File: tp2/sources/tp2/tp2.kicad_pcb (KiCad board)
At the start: 2 copper layers, 61.5 x 42 mm, 34 parts, among them Q1 NPN, U1 LM324, U7 LM324

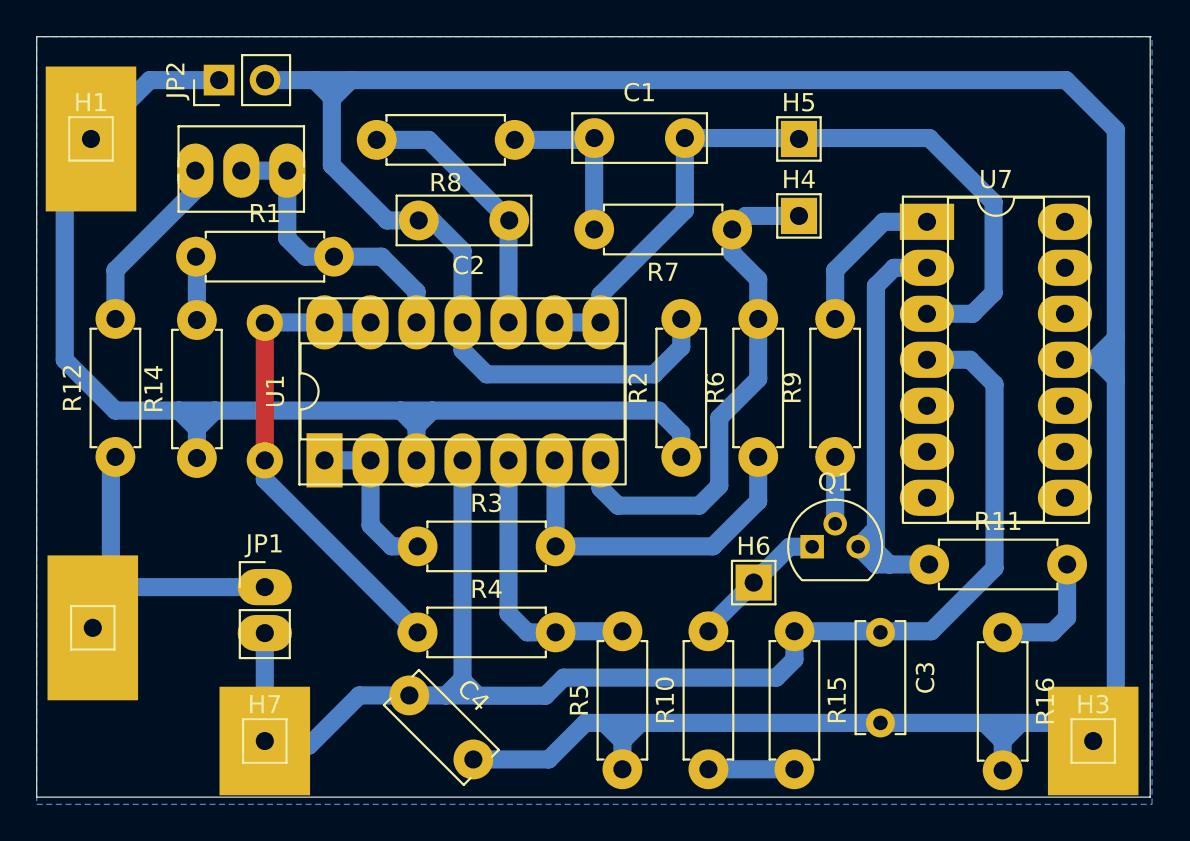
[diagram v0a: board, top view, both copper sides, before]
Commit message: tp2: achica 0.5mm (cero punto cinco milimietros) la placa
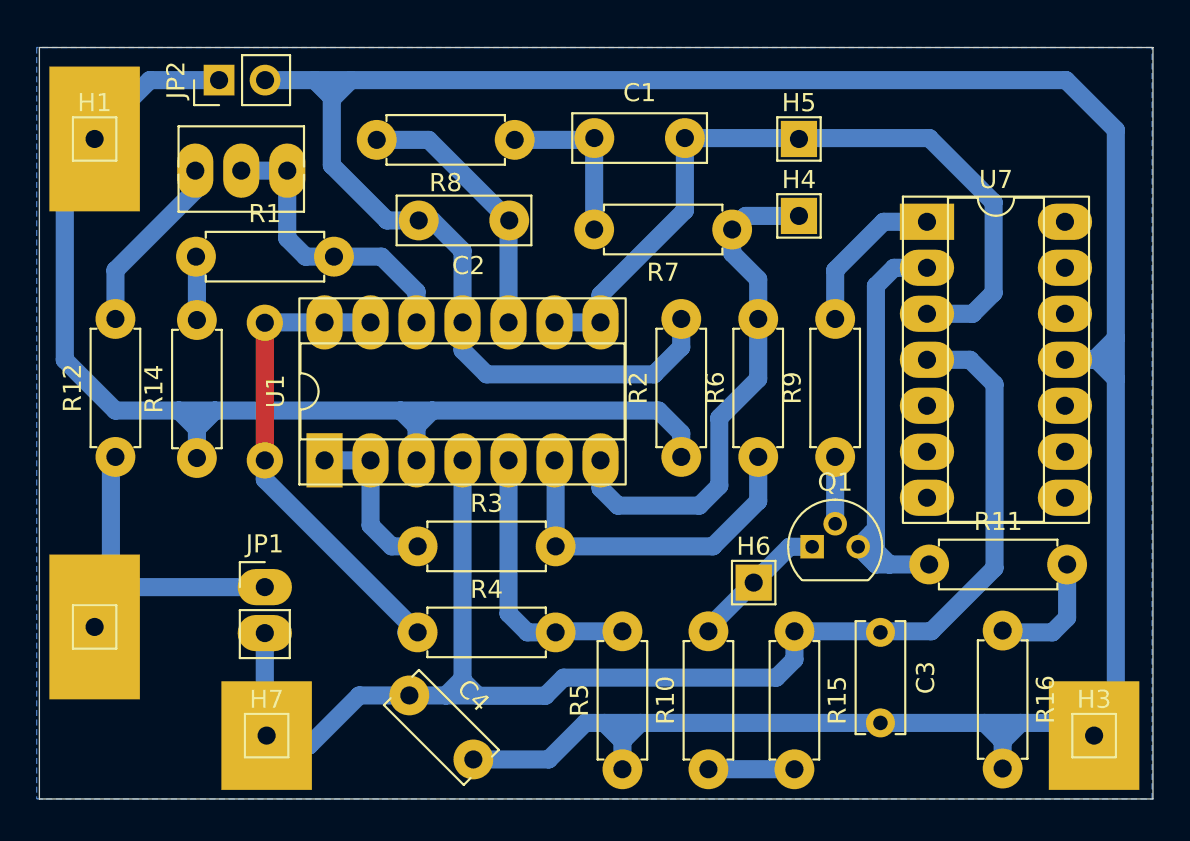
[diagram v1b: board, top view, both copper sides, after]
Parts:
- moved H7 0.32 mm to (107.6, 81.2)
- moved H3 0.30 mm to (153.3, 81.2)
- moved H1 0.20 mm to (98.1, 48.2)
- moved H2 0.11 mm to (98.1, 75.2)
- moved R16 0.10 mm to (148.2, 75.4)
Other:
- board size 61.5 x 42 mm -> 61.5 x 41.5 mm
